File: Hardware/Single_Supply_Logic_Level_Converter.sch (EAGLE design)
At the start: 23 parts, among them U1 TXB0104, U2 TPS61200, U4 MIC5219-3.3

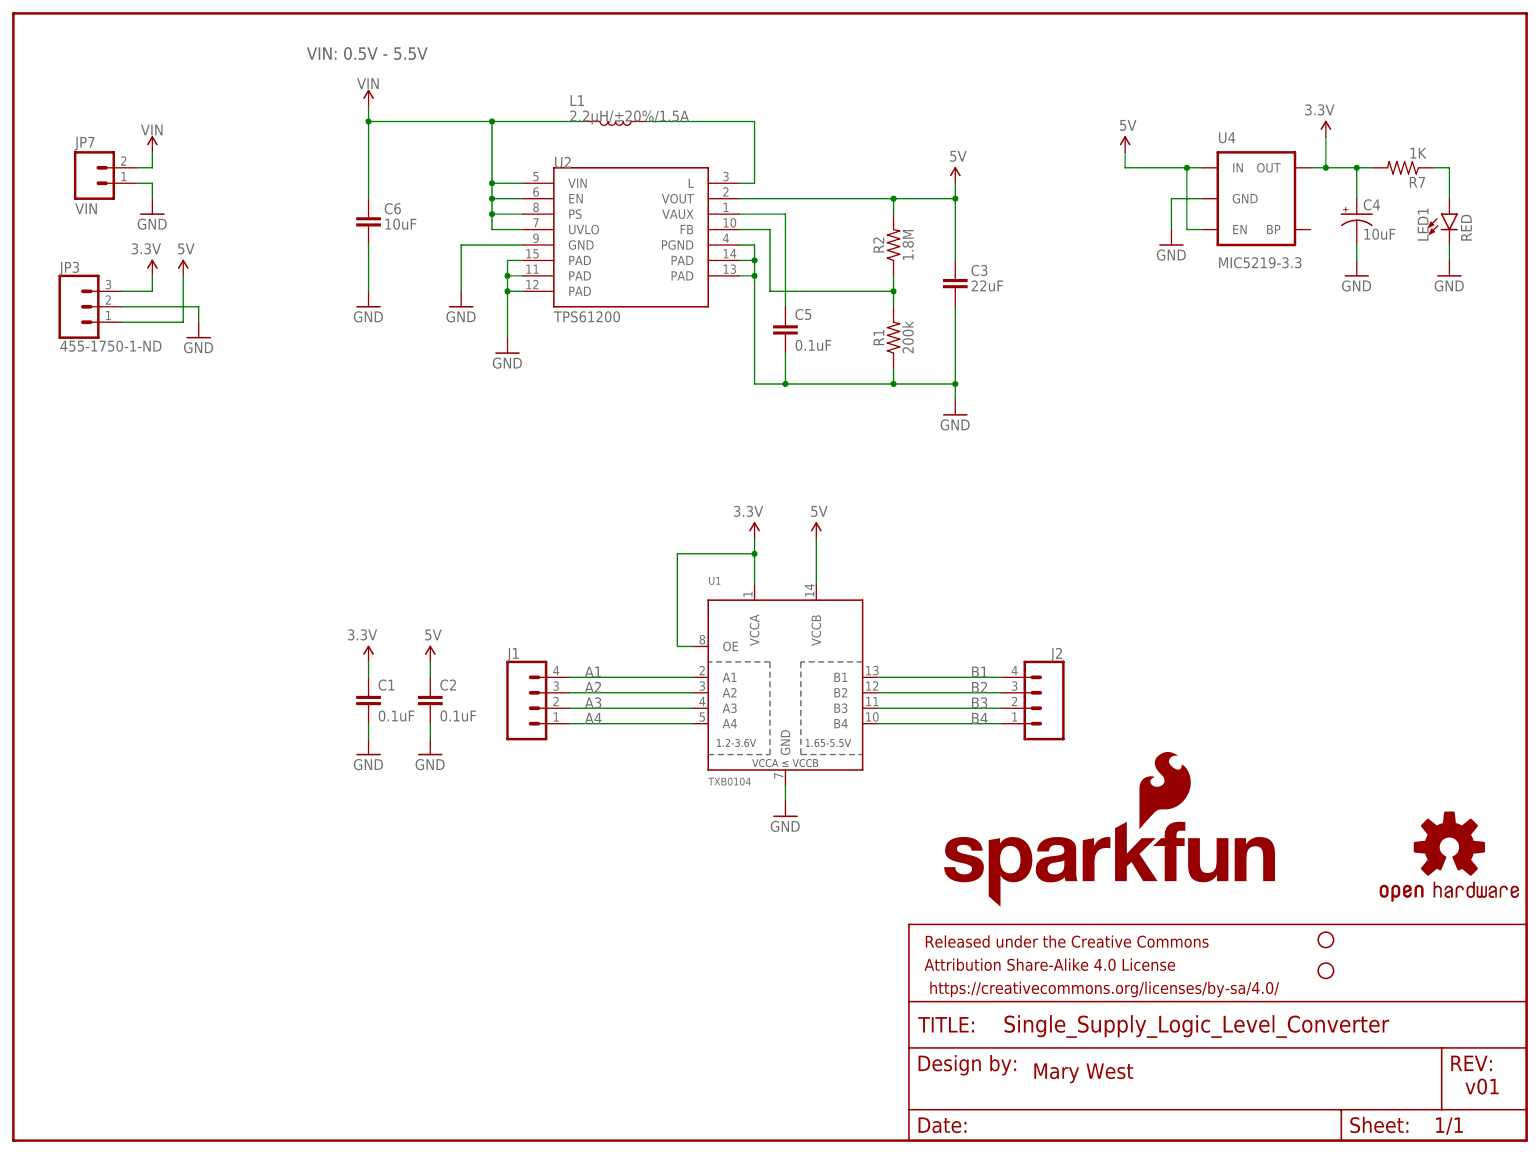
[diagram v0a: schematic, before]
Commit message: Updating design per review
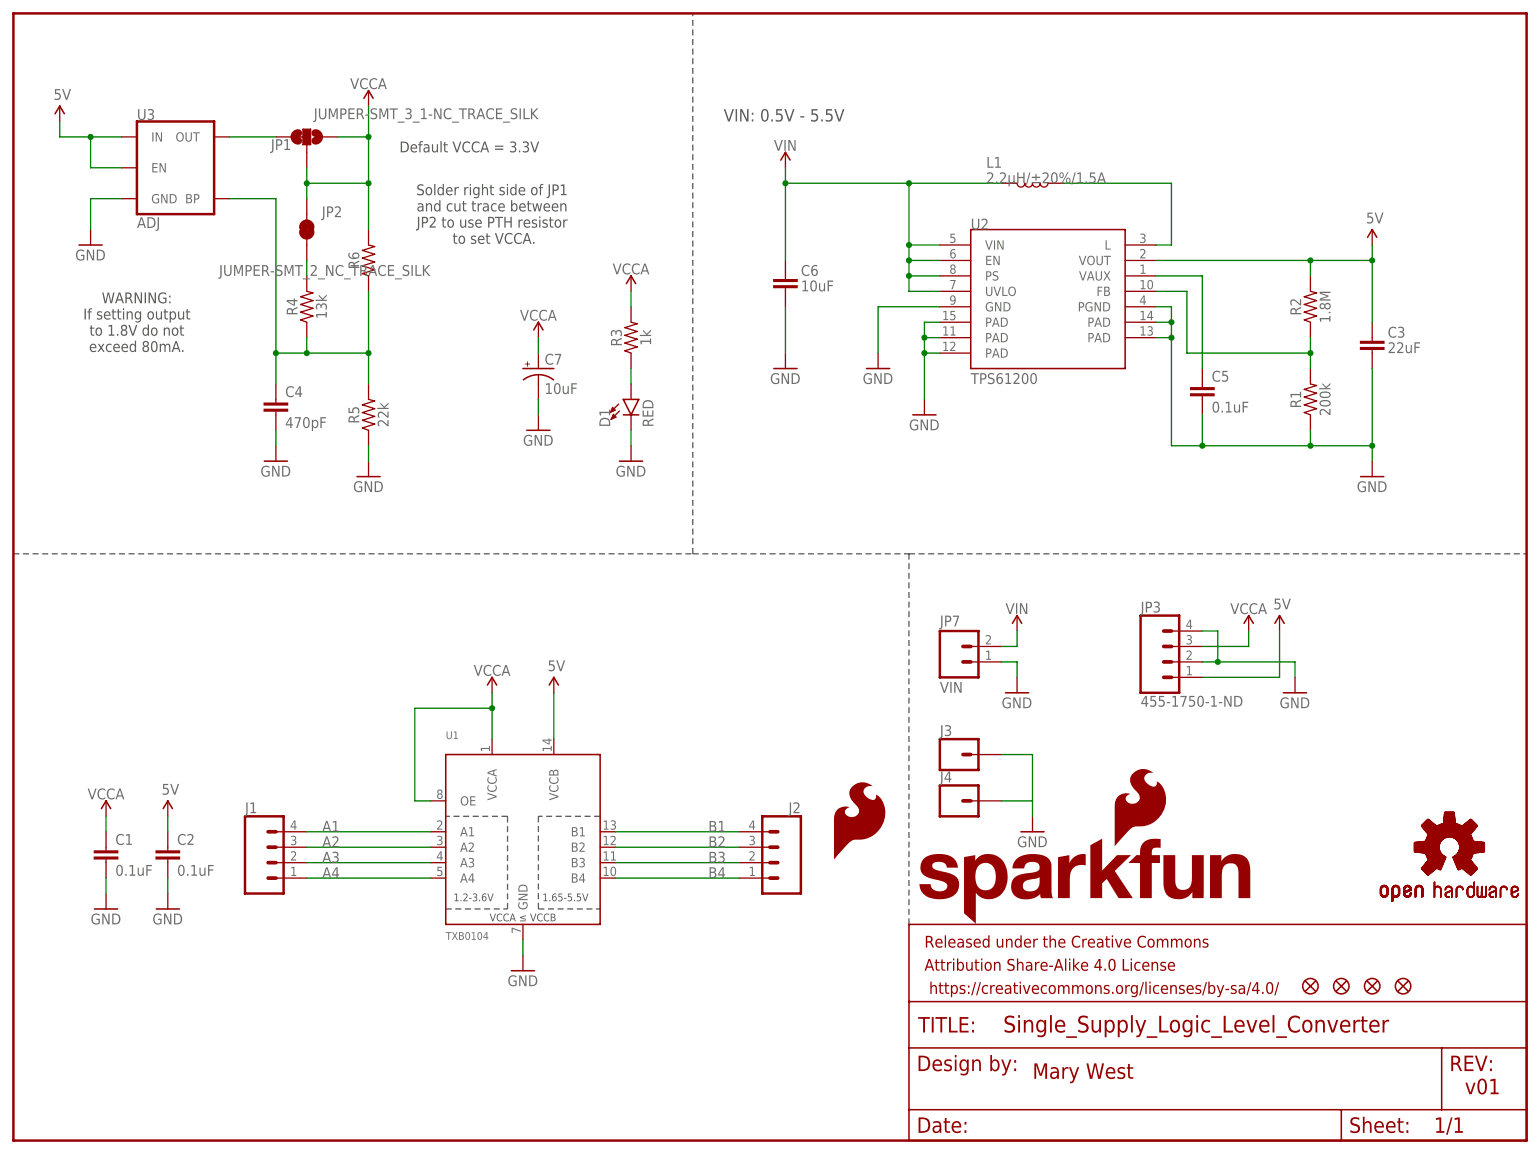
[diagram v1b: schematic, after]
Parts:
- removed H1, H2: STAND-OFFTIGHT, SparkFun-Hardware:STAND-OFFTIGHT
- removed LED1: RED, SparkFun-LED:LED-RED0603
- removed R7: 1K, SparkFun:RESISTOR0402-RES
- removed U4: MIC5219-3.3, SparkFun:V_REG_LDOSMD
- added C7: 10uF, SparkFun-Capacitors:10UF-POLAR-EIA3216-16V-10%(TANT)
- added D1: RED, SparkFun-LED:LED-RED0603
- added FD1, FD2, FD3, FD4: FIDUCIALUFIDUCIAL, SparkFun-Aesthetics:FIDUCIALUFIDUCIAL
- added J3, J4: (no value), SparkFun-Connectors:CONN_01
- added JP1: JUMPER-SMT_3_1-NC_TRACE_SILK, SparkFun-Jumpers:JUMPER-SMT_3_1-NC_TRACE_SILK
- added JP2: JUMPER-SMT_2_NC_TRACE_SILK, SparkFun-Jumpers:JUMPER-SMT_2_NC_TRACE_SILK
- added LOGO3: SFE_LOGO_FLAME.1_INCH, SparkFun-Aesthetics:SFE_LOGO_FLAME.1_INCH
- added LOGO4: OSHW-LOGOS, SparkFun-Aesthetics:OSHW-LOGOS
- added R3: 1k, SparkFun-Resistors:1KOHM-0603-1/10W-1%
- added R4: 13k, SparkFun-Resistors:13KOHM-0603-1/10W-1%
- added R5: 22k, SparkFun-Resistors:22KOHM-0603-1/10W-1%
- added R6: (no value), SparkFun-Resistors:RESISTORAXIAL-0.3
- added U3: ADJ, SparkFun-IC-Power:V_REG_MIC5205ADJ
- C4: value 10uF -> 470pF; device SparkFun:CAP_POL1206 -> SparkFun-Capacitors:470PF-0603-50V-5%
- C5: device SparkFun:CAP0603-CAP -> SparkFun-Capacitors:0.1UF-0603-25V-5%
- C6: device CH_passive:CAP1206 -> SparkFun-Capacitors:10UF-0603-6.3V-20%
- JP3: device SparkFun-Connectors:CONN_03 -> SparkFun-Connectors:CONN_04
- U2: device SparkFun:TPS61200 -> SparkFun-IC-Power:TPS61200
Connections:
- removed net 3.3V: C1.1, C4.+, JP3.3, R7.2, U1.OE, U1.VCCA, U4.OUT
- removed net N$4: LED1.A, R7.1
- new net N$1: JP1.3, U3.OUT
- new net N$11: C4.1, R4.1, R5.2, R6.1, U3.BP
- new net N$12: JP2.1, R4.2
- new net N$3: D1.A, R3.1
- new net VCCA: C1.1, C7.+, JP1.1, JP1.2, JP2.2, JP3.3, R3.2, R6.2, U1.OE, U1.VCCA
- net 5V: now also U3.EN, U3.IN; no longer U4.EN, U4.IN
- net GND: now also C4.2, C7.-, D1.C, J3.1, J4.1, JP3.4, R5.1, U3.GND; no longer C4.-, LED1.C, U4.GND
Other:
- note added: "Default VCCA = 3.3V"
- note added: "Solder right side of JP1 and cut trace between JP2 to use PTH resistor to set VCCA."
- note added: "WARNING: If setting output to 1.8V do not exceed 80mA."
- moved on the sheet: C1, C2, C3, C5, C6, J1, J2, JP7, L1, R1, R2, U1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
